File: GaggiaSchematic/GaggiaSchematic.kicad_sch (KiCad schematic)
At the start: 20 parts, among them J1 IEC_60320_C14_Receptacle, J2 cup Warmer GND, J3 chassis GND, K1 Relay_SPST-NO, K2 Relay_SPST-NO, SW2 Brew Switch, SW3 Steam Switch, SW4 power switch, U1 pressure sens, U2 ESP32-WROOM-32, U3 ThermoAmp

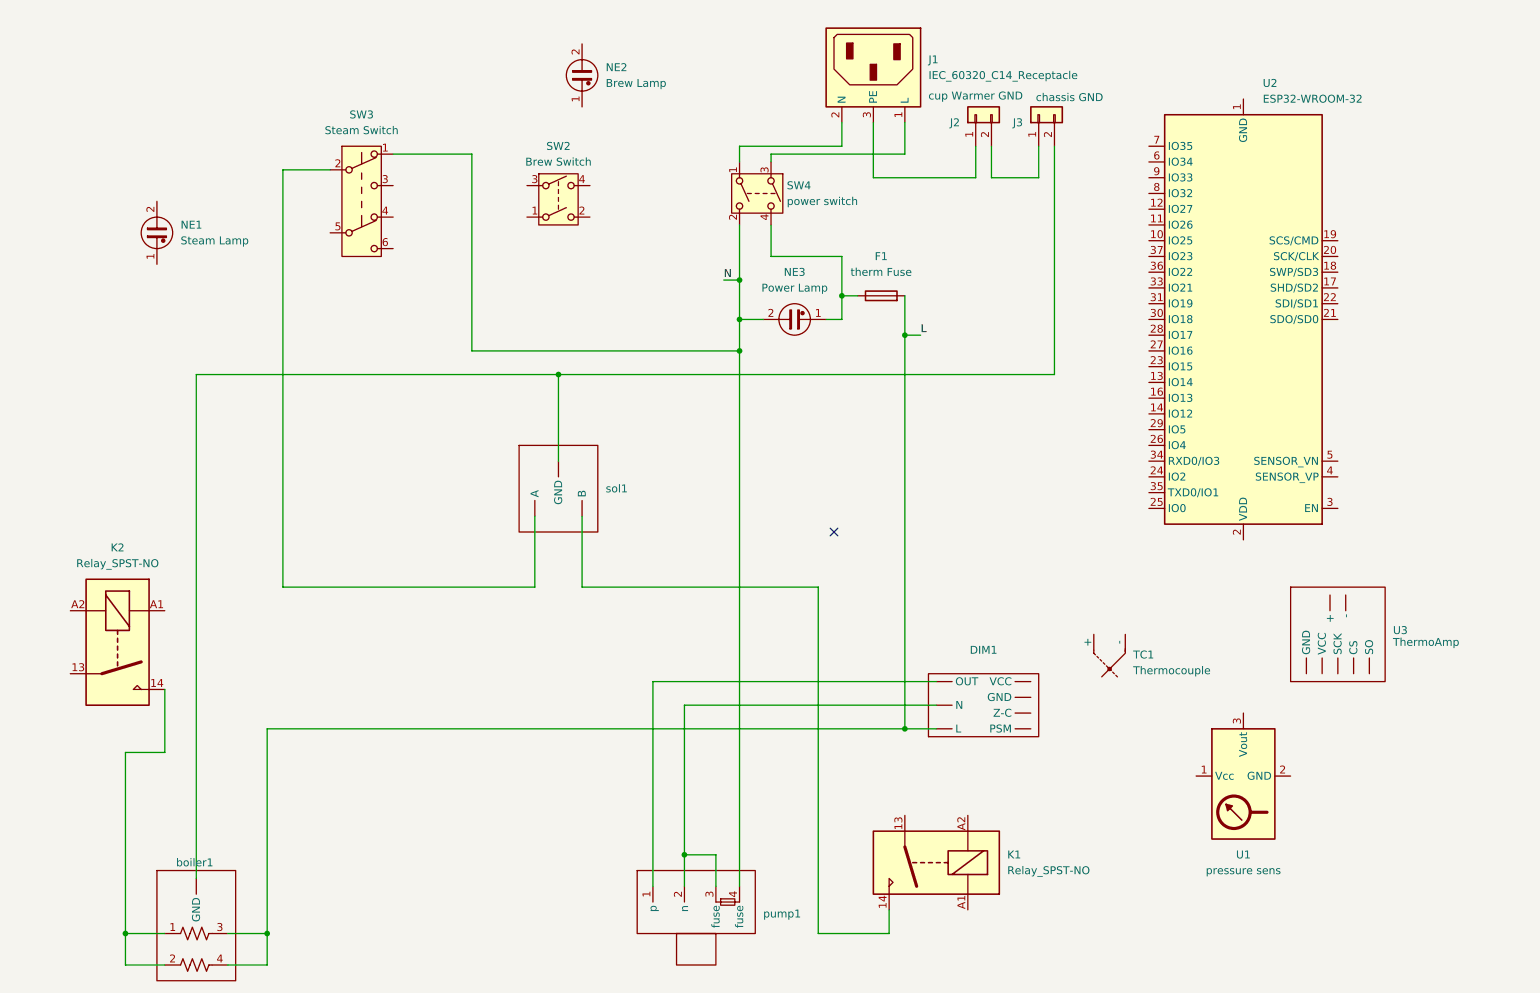
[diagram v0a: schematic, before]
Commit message: schematic v1
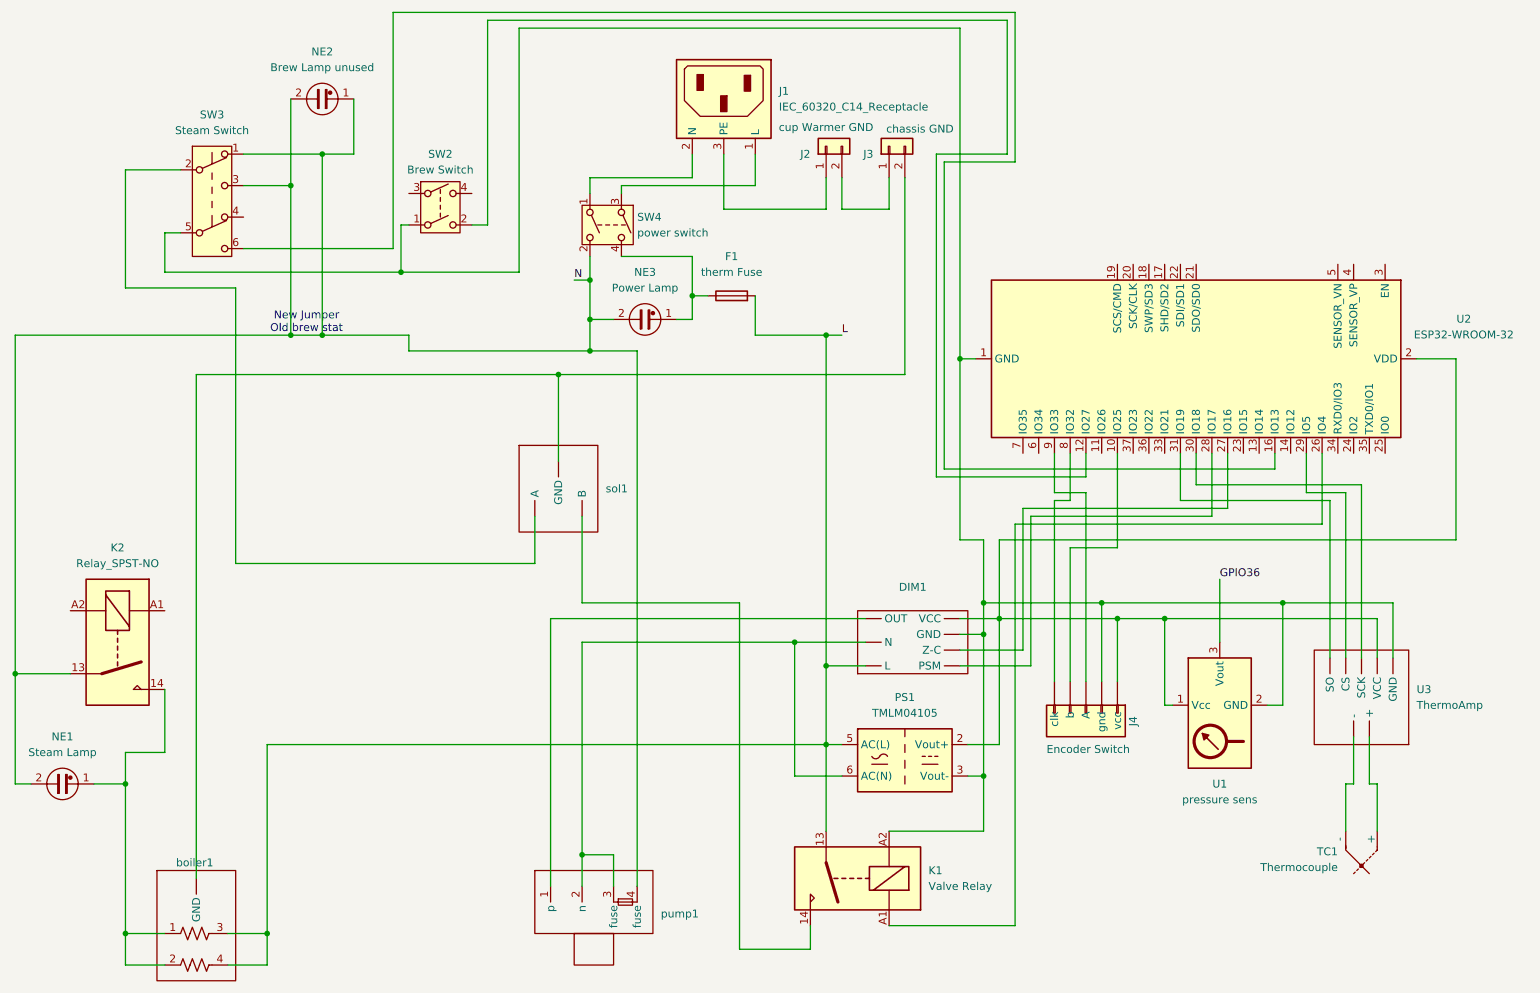
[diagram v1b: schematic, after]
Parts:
- added J4: Encoder Switch, symbol Connector_Generic:Conn_01x05
- added PS1: TMLM04105, Converter_ACDC:Converter_ACDC_TRACO_TMLM-04_THT, symbol Converter_ACDC:TMLM04105
- K1: value Relay_SPST-NO -> Valve Relay
- NE2: value Brew Lamp -> Brew Lamp unused
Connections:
- net L: now also K1.13, PS1.5 (AC(L))
- net N: now also K2.13, NE1.2, NE2.1, NE2.2, SW3.3 (C)
- net at U2.1 (GND), U2.15 (GND), U2.38 (GND)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: now also DIM1. (VCC), K1.A2, SW2.1, SW3.5 (B), U1.2 (GND), U3. (SO), J4.2 (gnd), PS1.3 (Vout-)
- net at U2.10 (IO25): now also J4.4 (b)
- net at U2.12 (IO27): now also SW2.2
- net at U2.16 (IO13): now also SW3.6 (C)
- net at U2.2 (VDD): now also DIM1. (VCC), U1.1 (Vcc), U3. (SO), J4.1 (vcc), PS1.2 (Vout+)
- net at U2.26 (IO4): now also K1.A1
- net at U2.27 (IO16): now also DIM1. (VCC)
- net at U2.28 (IO17): now also DIM1. (VCC)
- net at U2.29 (IO5): now also U3. (SO)
- net at U2.30 (IO18): now also U3. (SO)
- net at U2.31 (IO19): now also U3. (SO)
- net at U2.8 (IO32): now also J4.5 (clk)
- net at U2.9 (IO33): now also J4.3 (A)
- net at K2.14, boiler1.1, boiler1.2: now also NE1.1
- net GPIO36: now reaches U1.3 (Vout)
- net at DIM1. (VCC), pump1.2 (n), pump1.3 (fuse): now also PS1.6 (AC(N))
- net at U3. (SO): now also TC1.2 (-)
- net at TC1.1 (+): now also U3. (SO)
- no-connect marks 1 -> 0
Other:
- note added: "New Jumper Old brew stat"
- moved on the sheet: DIM1, F1, J1, J2, J3, K1, NE1, NE2, NE3, SW2, SW3, SW4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
